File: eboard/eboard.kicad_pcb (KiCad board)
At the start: 4 copper layers, 87 x 87 mm, 103 parts, among them J1 Conn_01x02_Male, J11 Conn_01x02_Male, J12 Conn_01x02_Male, J13 Conn_01x02_Male, J14 Conn_01x02_Male, J15 Conn_01x02_Male, J16 Conn_01x03_Male, J17 Conn_01x03_Male, J18 Conn_01x03_Male, J19 Conn_01x03_Male, J2 USB_B_Micro, J20 Conn_01x02_Male, J21 Conn_01x02_Male, J3 Conn_01x03_Male, J4 jst_battery, J5 Conn_01x02_Male, J7 Conn_01x04_Male, J9 Conn_01x06_Male, Q1 AO4407, Q10 BSS138K, Q11 AO4407, Q12 BSS138K, Q13 BSS138K, Q14 BSS138K, Q15 BSS138K, Q16 BSS138K, Q17 BSS138K, Q18 AO4407, Q19 AO4407, Q2 S8050, Q20 AO4407, Q3 S8050, Q9 BSS138K, SW1 pushbutton_switch, SW2 pushbutton_switch, U1 ESP32-PICO-D4, U2 TPS63000, U3 TP4056, U4 SRV05-4, U5 CP2102, U7 SRV05-4, U8 SRV05-4, U9 SRV05-4

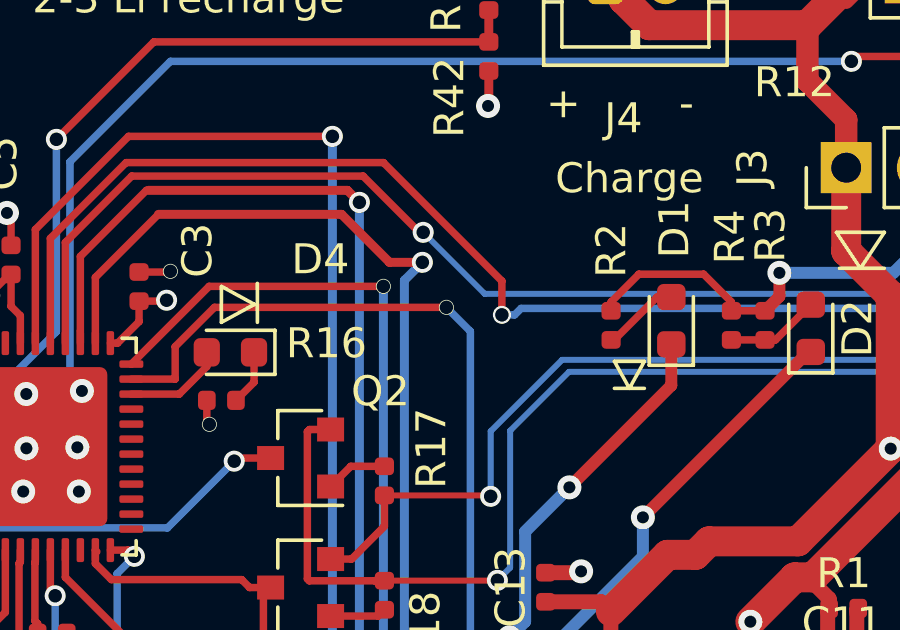
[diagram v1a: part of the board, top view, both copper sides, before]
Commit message: leds
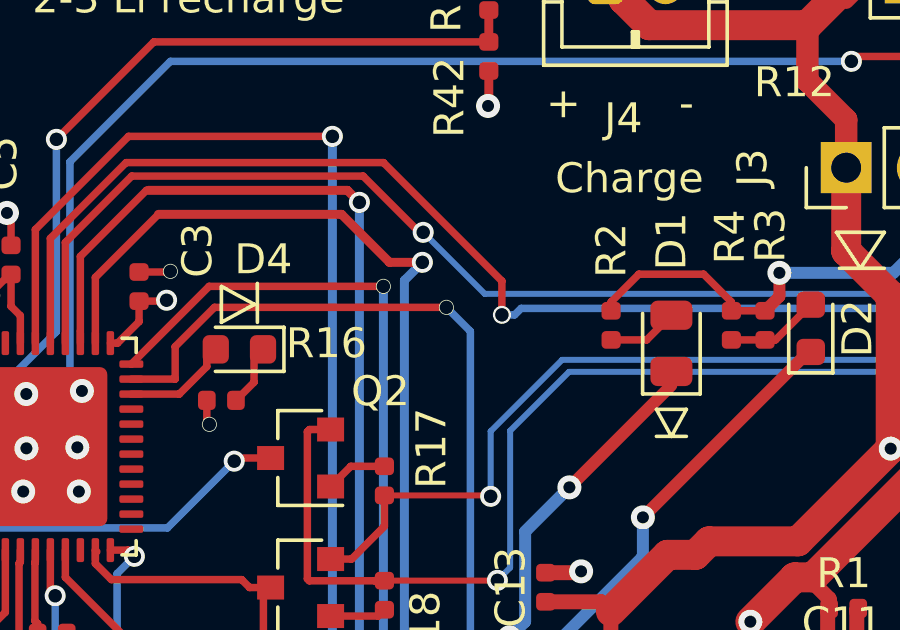
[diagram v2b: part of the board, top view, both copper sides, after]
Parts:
- D1: value ledgreen -> ledgreen_0805; footprint LED_SMD:LED_0603_1608Metric -> LED_SMD:LED_0805_2012Metric
- D4: value ledgreen -> ledyellow
- moved D1 0.76 mm to (78.4, 45.2)
- moved D4 0.32 mm to (64.0, 45.4)
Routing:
- net nCHRG: track 17.1 -> 15.7 mm
